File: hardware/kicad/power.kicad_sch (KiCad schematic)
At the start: 23 parts, among them Q1 DMG3415UQ-7, Q2 PMV32UP, Q7 DMG1012UW, U10 RT9080-33GJ5, U12 RT9193, U3 TPS22917DBVR, U8 XC6215B332MR-G

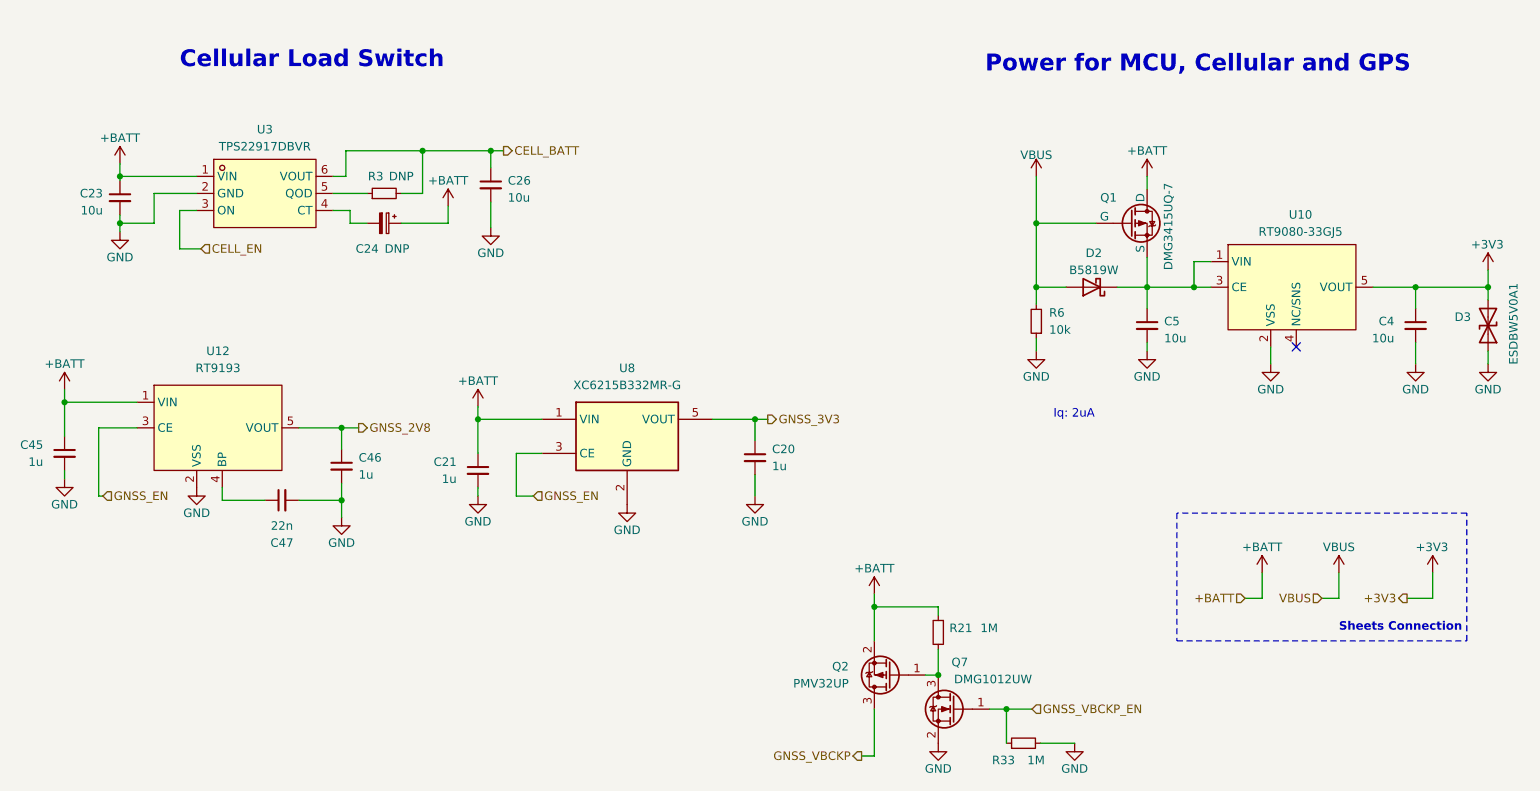
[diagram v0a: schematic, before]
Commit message: wip: revision 2
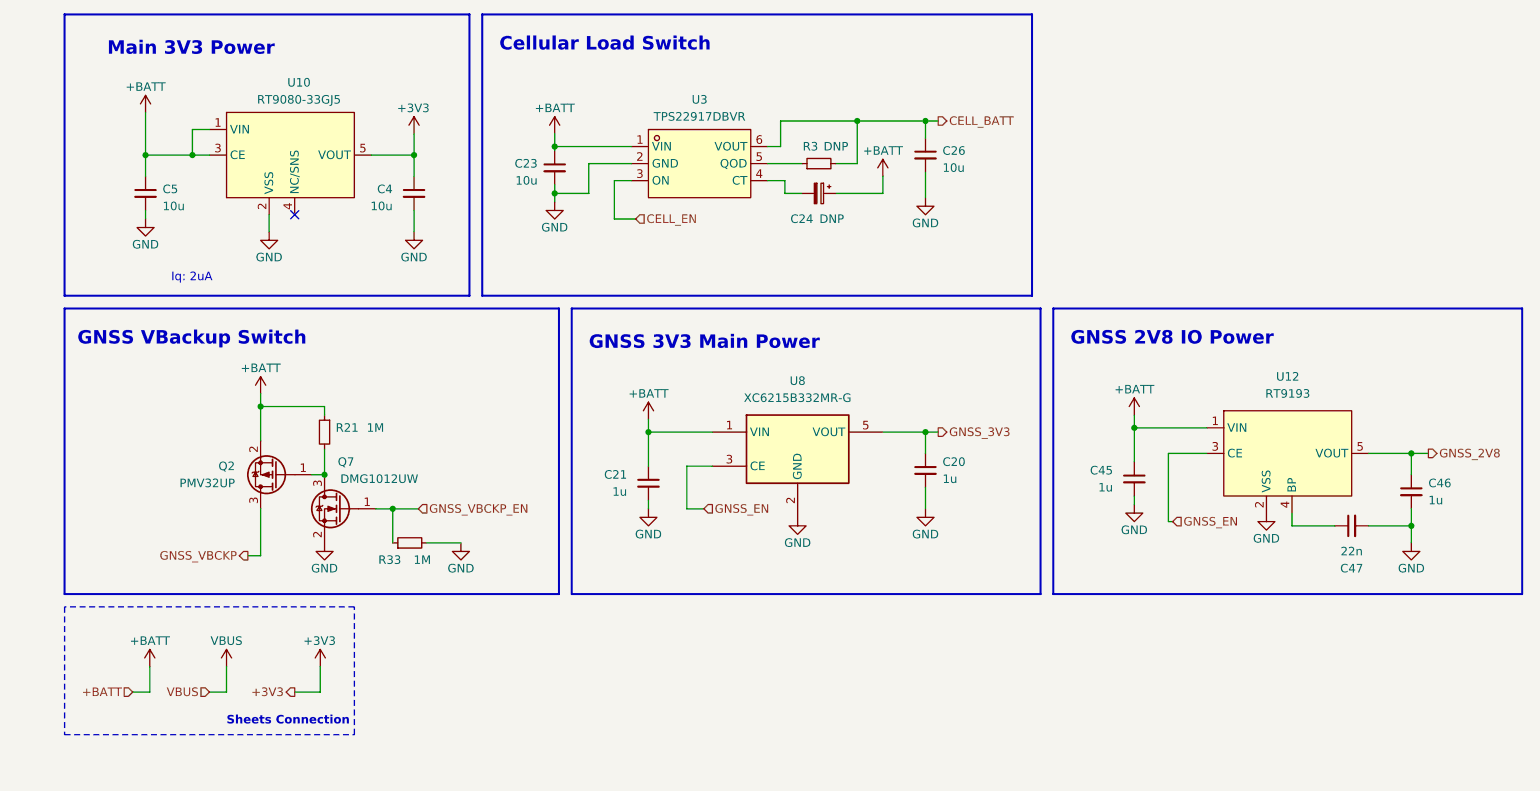
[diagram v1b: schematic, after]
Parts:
- removed D2: B5819W, Diode_SMD:D_SOD-123, symbol Device:D_Schottky
- removed D3: ESDBW5V0A1, Capacitor_SMD:C_0402_1005Metric, symbol Device:D_TVS
- removed Q1: DMG3415UQ-7, Package_TO_SOT_SMD:SOT-23, symbol Simulation_SPICE:PMOS
- removed R6: 10k, Resistor_SMD:R_0402_1005Metric, symbol Device:R_Small
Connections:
- net +BATT: now also C5.1, U10.1 (VIN), U10.3 (CE)
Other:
- note added: "GNSS 2V8 IO Power"
- note added: "GNSS 3V3 Main Power"
- note added: "GNSS VBackup Switch"
- note added: "Main 3V3 Power"
- note removed: "Power for MCU, Cellular and GPS"
- moved on the sheet: C20, C21, C23, C24, C26, C4, C45, C46, C47, C5, Q2, Q7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

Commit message: wip: revision 2
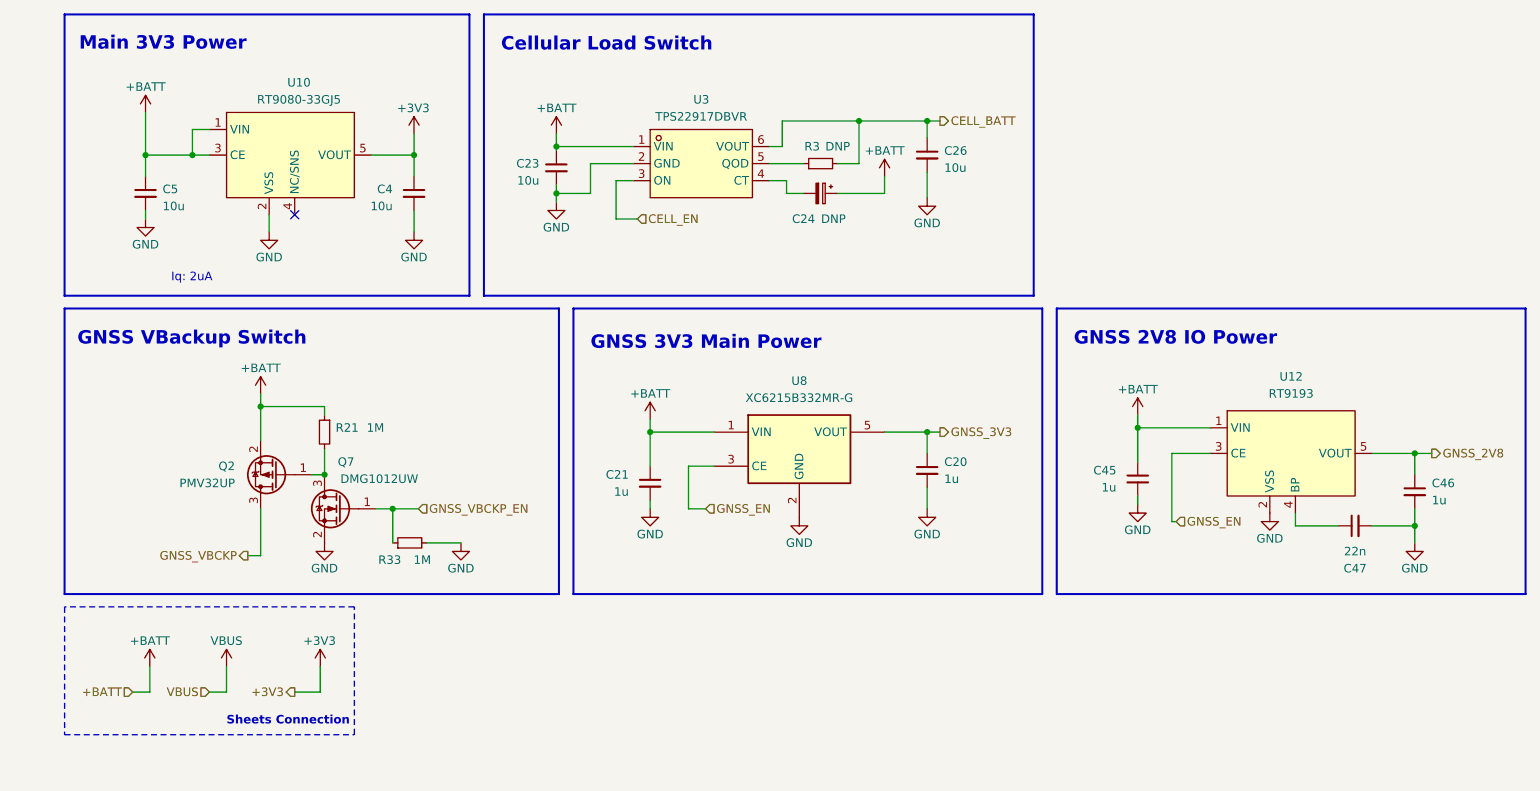
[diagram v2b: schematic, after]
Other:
- moved on the sheet: C45, C46, C47, U12
